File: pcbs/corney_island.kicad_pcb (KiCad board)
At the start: 2 copper layers, 133.8 x 91.7 mm, 101 parts

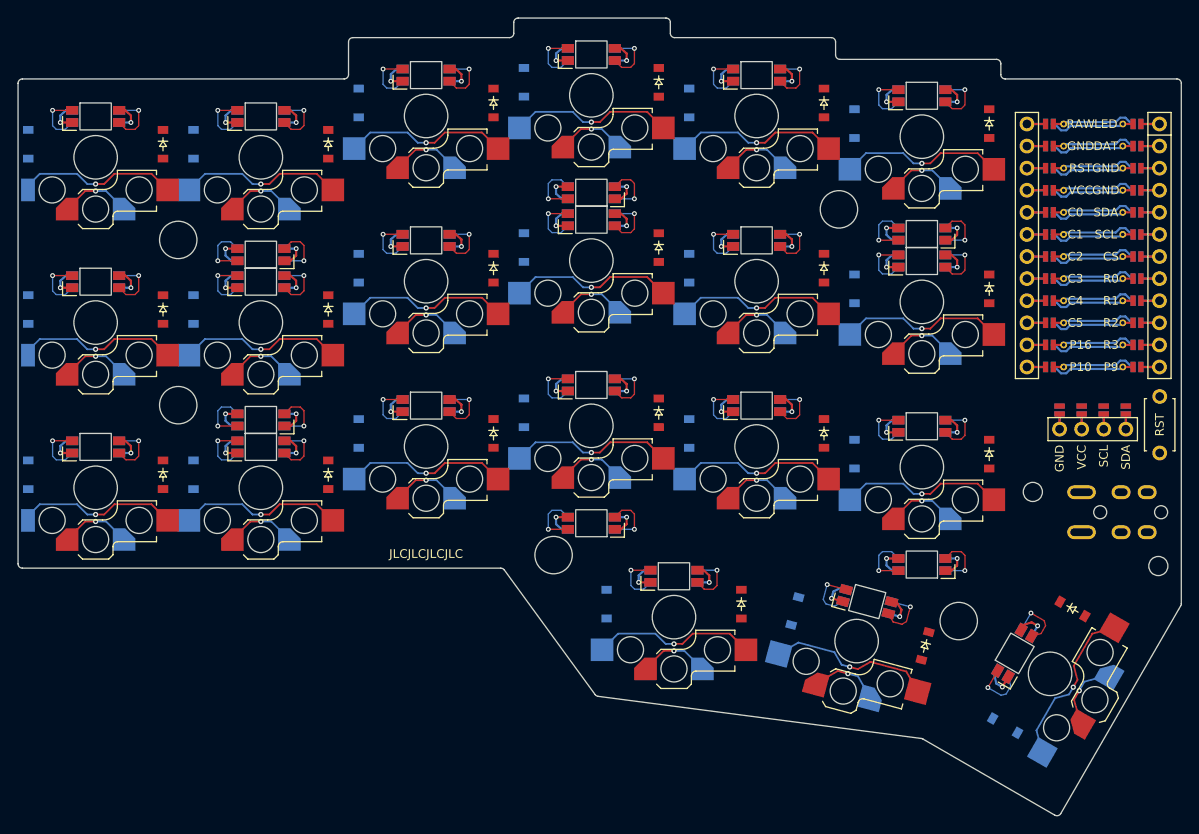
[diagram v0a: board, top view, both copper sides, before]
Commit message: build: regenerate outlines and PCBs with Ergogen snapshot
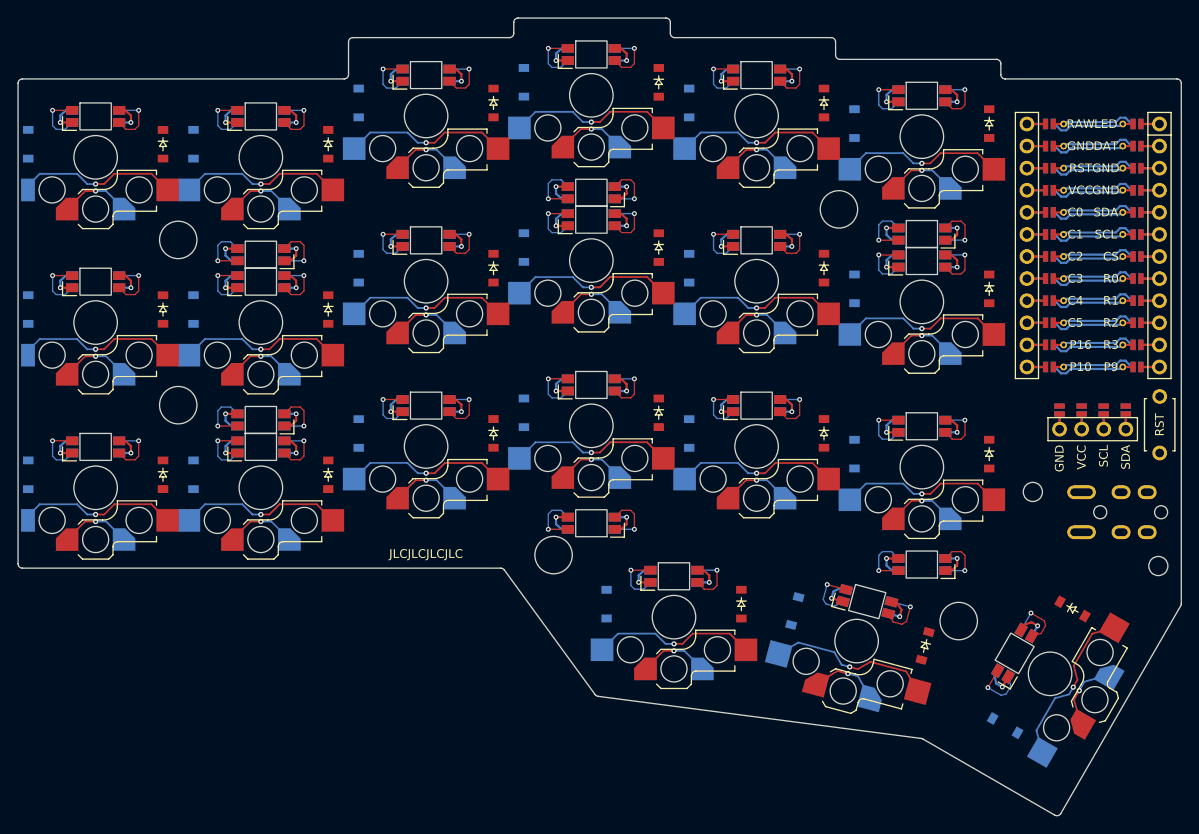
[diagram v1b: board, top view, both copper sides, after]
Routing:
- net (no net): track 0.00 -> 333.1 mm
- net GND: track 130.3 -> 101.4 mm
- net C5: track 42.7 -> 33.1 mm
- net C3: track 42.7 -> 33.1 mm
- net C1: track 34.5 -> 24.8 mm
- net RST: track 9.64 -> 0.00 mm
- net RAW: track 9.64 -> 0.00 mm
- net C2: track 34.5 -> 24.8 mm
- net P16: track 9.64 -> 0.00 mm
- net C0: track 34.5 -> 24.8 mm
- net P10: track 9.64 -> 0.00 mm
- net C4: track 42.7 -> 33.1 mm
- net VCC: track 111.0 -> 101.4 mm
- net SDA: track 9.63 -> 0.00 mm
- net R3: track 9.63 -> 0.00 mm
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
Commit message: build: regenerate PCBs, images, and gerbers
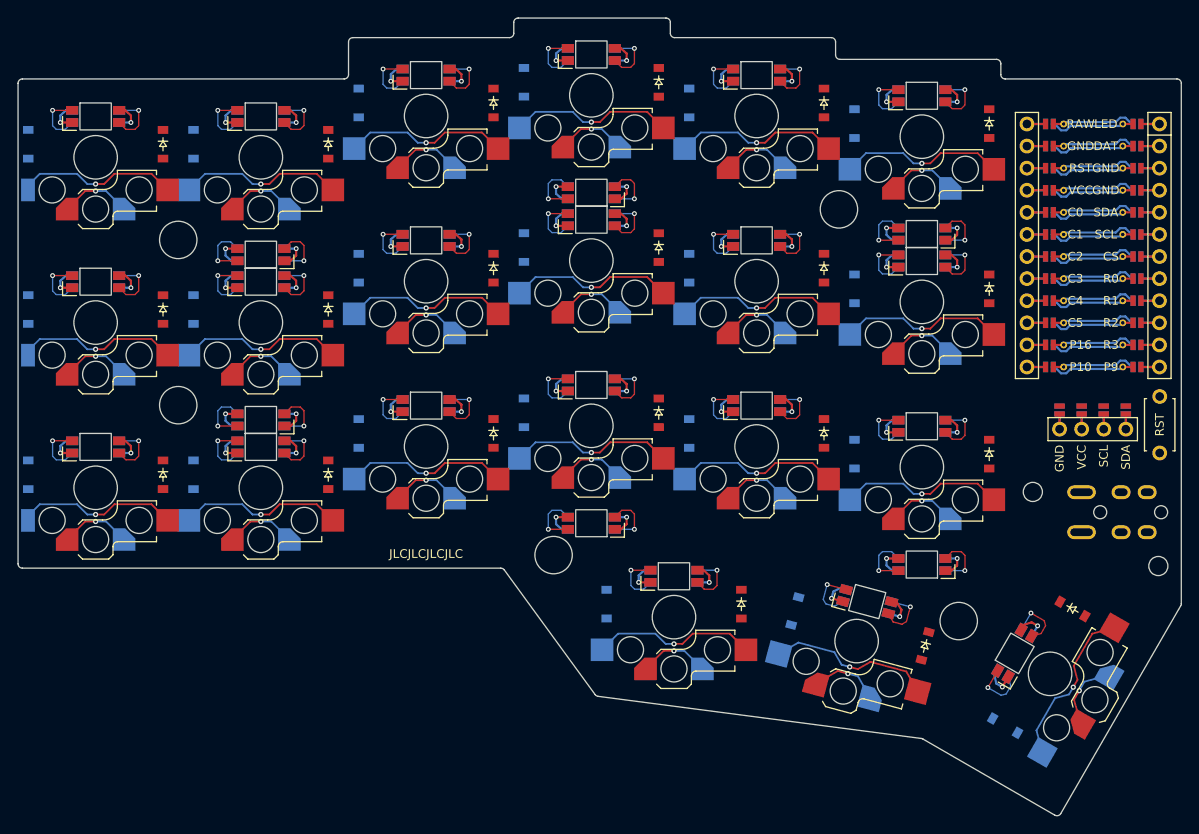
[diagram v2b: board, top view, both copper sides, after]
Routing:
- net (no net): track 333.1 -> 0.00 mm
- net GND: track 101.4 -> 130.3 mm
- net C5: track 33.1 -> 42.7 mm
- net C3: track 33.1 -> 42.7 mm
- net C1: track 24.8 -> 34.5 mm
- net RST: track 0.00 -> 9.64 mm
- net RAW: track 0.00 -> 9.64 mm
- net C2: track 24.8 -> 34.5 mm
- net P10: track 0.00 -> 9.64 mm
- net C0: track 24.8 -> 34.5 mm
- net P16: track 0.00 -> 9.64 mm
- net C4: track 33.1 -> 42.7 mm
- net VCC: track 101.4 -> 111.0 mm
- net SDA: track 0.00 -> 9.63 mm
- net R3: track 0.00 -> 9.63 mm
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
